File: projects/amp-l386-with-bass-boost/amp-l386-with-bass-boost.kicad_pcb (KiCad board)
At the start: 2 copper layers, 78 x 60.1 mm, 22 parts, among them U1 LM386

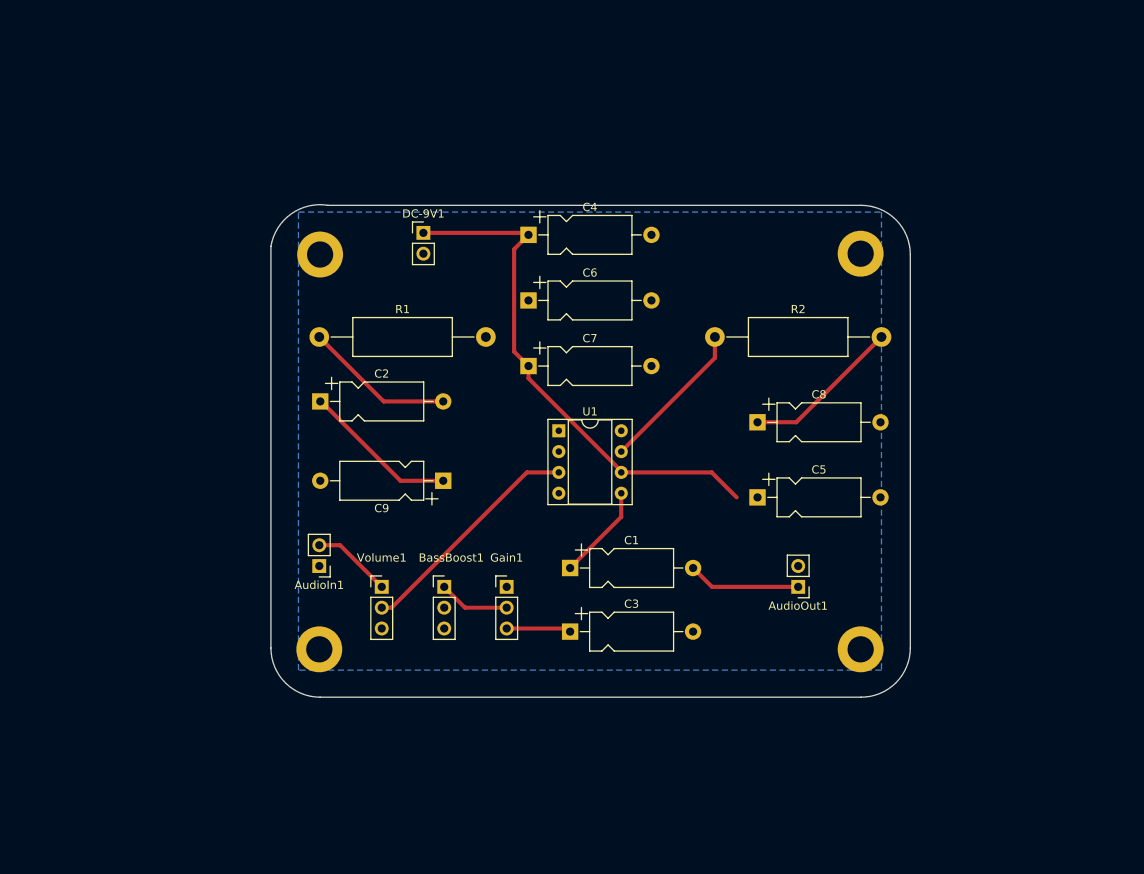
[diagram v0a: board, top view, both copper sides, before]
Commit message: Incremental changes optimizing PCB layout
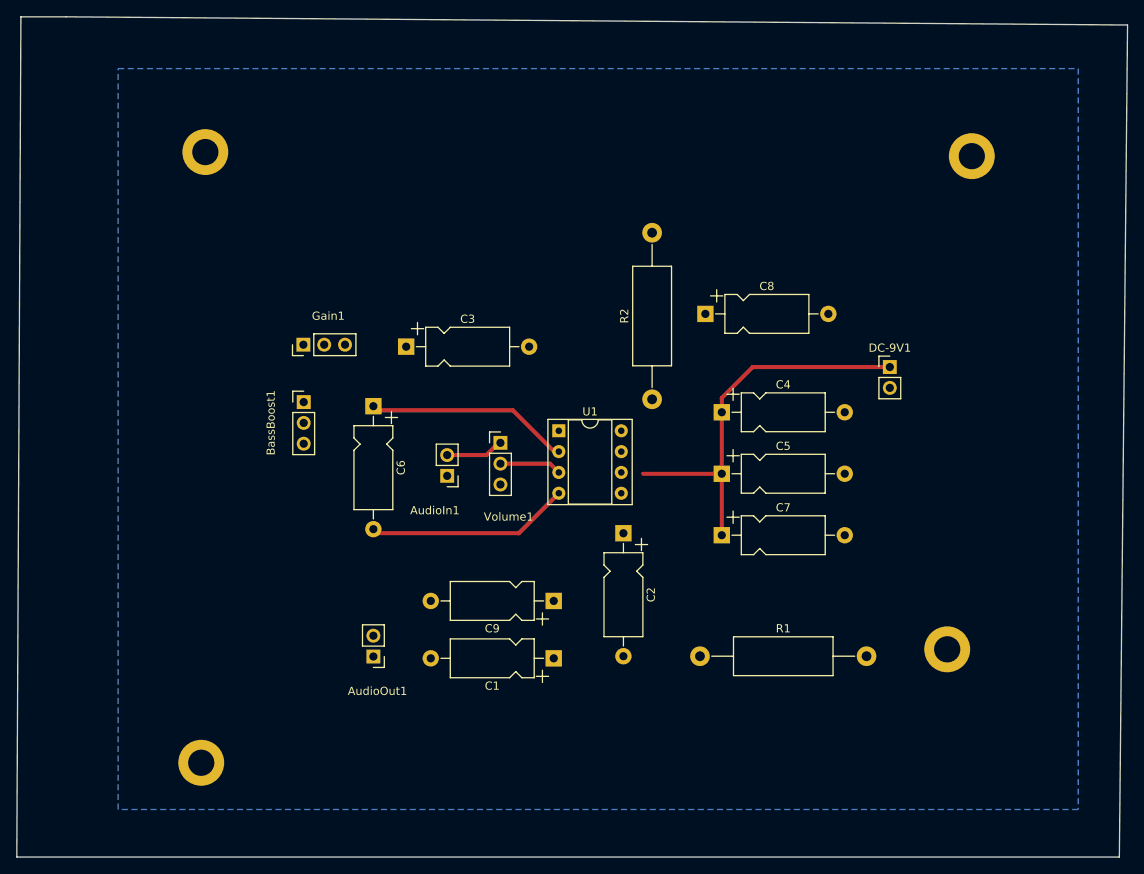
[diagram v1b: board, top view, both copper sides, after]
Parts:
- C6: value 470pF -> 470pF w/2&4
- moved R1 60.6 mm to (135.3, 138.0)
- moved DC-9V1 59.2 mm to (158.5, 102.7)
- moved AudioOut1 52.5 mm to (95.5, 138.0)
- moved C2 40.3 mm to (126.0, 123.0), turned to -90 degrees
- moved C3 40.1 mm to (99.5, 100.2)
- moved Gain1 38.6 mm to (87.0, 100.0), turned to 90 degrees
- moved C4 32.0 mm to (138.0, 108.2)
- moved C7 31.3 mm to (138.0, 123.2)
- moved BassBoost1 28.3 mm to (87.0, 107.0)
- moved C6 22.9 mm to (95.5, 107.5), turned to -90 degrees
- moved Volume1 22.8 mm to (111.0, 112.0)
- moved H1 20.0 mm to (74.5, 151.0)
- moved C9 19.9 mm to (117.5, 131.3)
- moved AudioIn1 19.1 mm to (104.5, 116.0)
- moved H4 18.8 mm to (75.0, 76.5)
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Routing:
- net GND: track 0.00 -> 49.8 mm
- net Net-(C1-Pad1): track 30.9 -> 0.00 mm
- net Net-(U1-Pad3): track 28.4 -> 7.56 mm
- net Net-(C8-Pad1): track 19.4 -> 0.00 mm
- net Net-(R2-Pad1): track 18.7 -> 0.00 mm
- net Net-(C2-Pad2): track 18.4 -> 0.00 mm
- net +9V: track 63.4 -> 49.2 mm
- net Net-(AudioOut1-Pad1): track 13.8 -> 0.00 mm
- net Net-(BassBoost1-Pad1): track 8.67 -> 0.00 mm
- net Net-(C3-Pad1): track 7.90 -> 0.00 mm
- net Net-(AudioIn1-PadT): track 9.72 -> 7.12 mm
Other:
- board size 78 x 60.1 mm -> 135.5 x 102.5 mm
